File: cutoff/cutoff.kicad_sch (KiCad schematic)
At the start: 31 parts, among them J1 Conn_01x01, J10 Conn_01x01, J11 Conn_01x01, J12 Conn_01x01, J13 Conn_01x01, J14 Conn_01x01, J15 Conn_01x01, J2 Conn_01x01, J3 Conn_01x01, J4 Conn_01x01, J5 Conn_01x01, J6 Conn_01x01, J7 Conn_01x01, J8 Conn_01x01, J9 Conn_01x01, U1 TPS3700DDCR, U2 BTS50010-1TAD

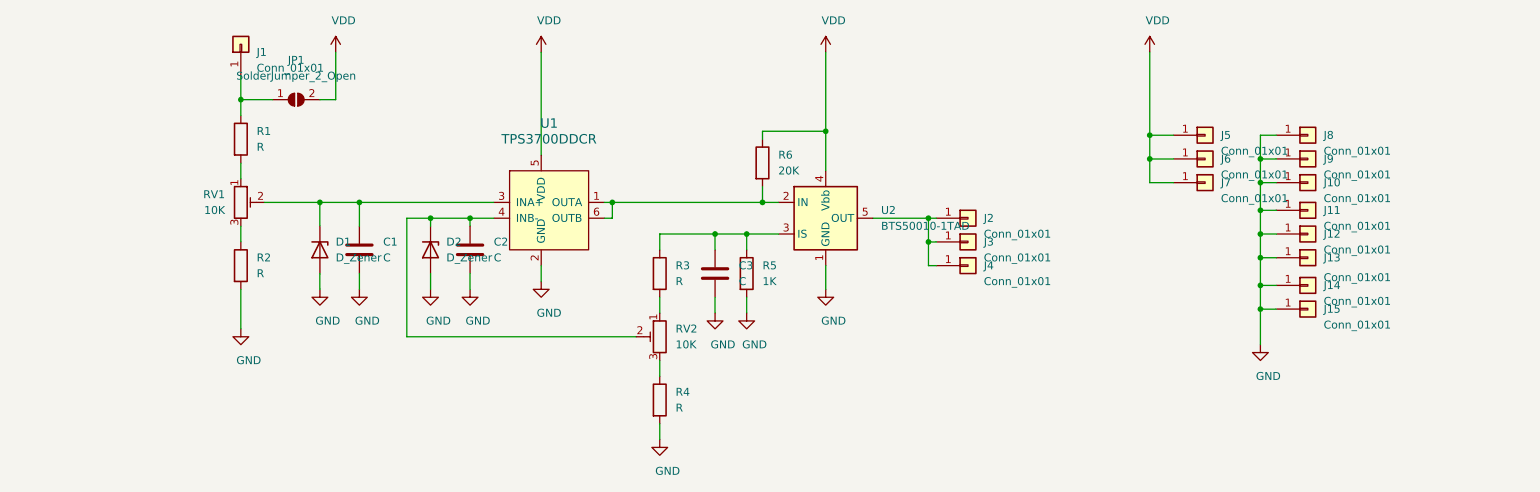
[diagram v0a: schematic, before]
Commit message: .
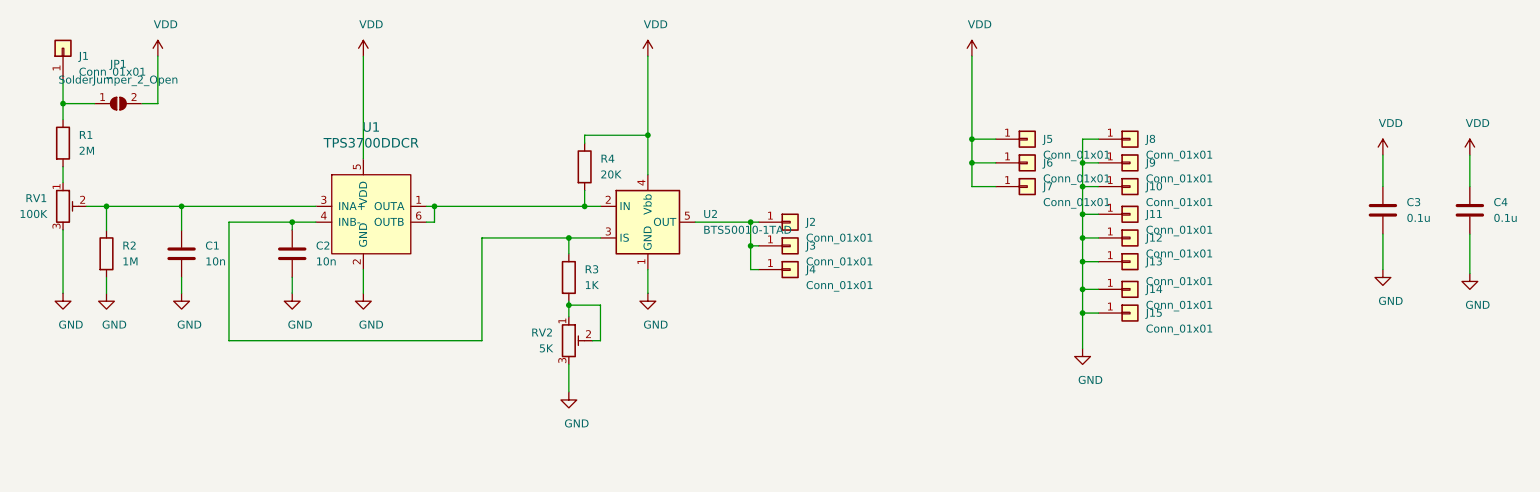
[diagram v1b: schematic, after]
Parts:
- removed D1, D2: D_Zener, Diode_SMD:D_1206_3216Metric_Pad1.42x1.75mm_HandSolder, symbol Device:D_Zener
- removed R3, R4: R, Resistor_SMD:R_0805_2012Metric_Pad1.20x1.40mm_HandSolder, symbol Device:R
- added C4: 0.1u, Capacitor_SMD:C_0805_2012Metric_Pad1.18x1.45mm_HandSolder, symbol Device:C
- C1, C2: value C -> 10n
- C3: value C -> 0.1u
- R1: value R -> 2M
- R2: value R -> 1M
- RV1: value 10K -> 100K
- RV2: value 10K -> 5K
- renumbered R5 to R3, R6 to R4
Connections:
- net GND: now also RV1.3, RV2.3, C4.2; no longer R3.2
- net VDD: now also C3.1, C4.1
- net at C1.1, RV1.2, U1.3 (INA+): now also R2.1
- net at R3.1, U2.3 (IS): now also C2.1, U1.4 (INB-); no longer C3.1
- net at RV2.1: now also R3.2, RV2.2
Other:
- moved on the sheet: C1, C2, J1, J10, J11, J12, J13, J14, J15, J2, J3, J4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
